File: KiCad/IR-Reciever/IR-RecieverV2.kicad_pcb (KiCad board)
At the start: 2 copper layers, 19.7 x 17.8 mm, 6 parts, among them P1 CONN_6, U1 TSOP38238, U2 TSOP38238, U3 TSOP38238, U4 RGBLED

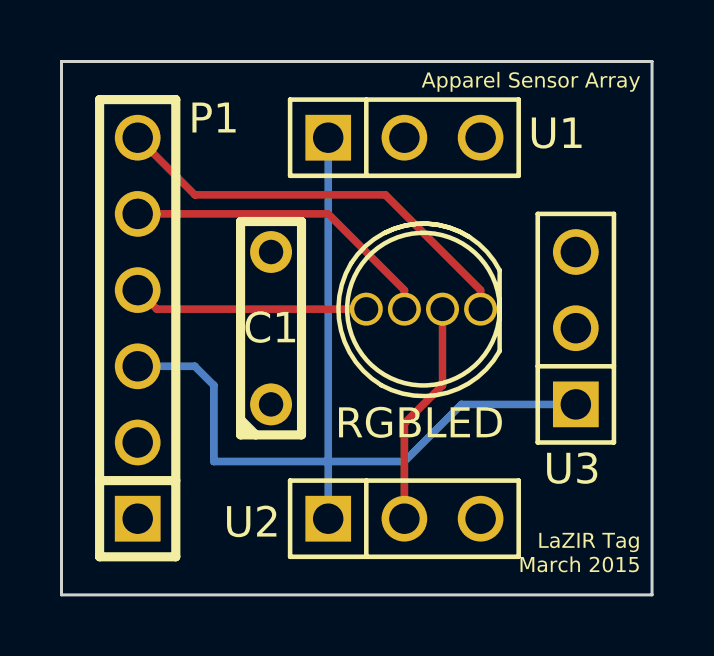
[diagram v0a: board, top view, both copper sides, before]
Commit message: Revert "Revert "3/29 KiCad Updates""
This reverts commit 46467126b97e8d3ee2ff82587e11af580e6d6854.
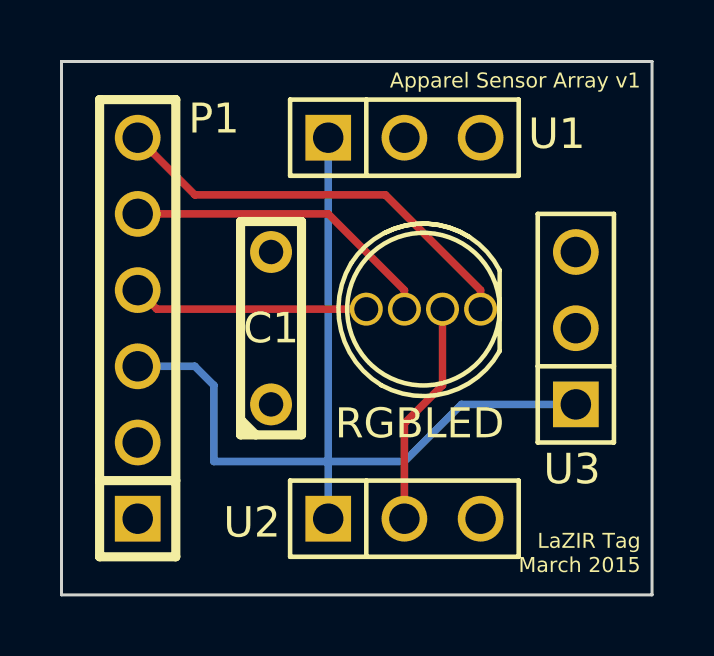
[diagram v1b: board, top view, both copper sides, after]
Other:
- board text added: "Apparel Sensor Array v1"
- board text removed: "Apparel Sensor Array"
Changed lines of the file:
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@@
     )
   )
-  (gr_text "Apparel Sensor Array" (at 45.974 22.86) (layer F.SilkS)
+  (gr_text "Apparel Sensor Array v1" (at 45.974 22.86) (layer F.SilkS)
     (effects (font (size 0.5 0.5) (thickness 0.125)) (justify right))
   )
